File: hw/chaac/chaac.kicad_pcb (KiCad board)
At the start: 4 copper layers, 53 parts, among them J1 Battery, J2 TC2030-CTX, J3 UART, J4 windrain, Q1 Q_PMOS_GSD, SW1 RST, SW2 RST, U1 TPS7A0530PDBVT, U2 NRF52811-QFAA, U3 BMP280, U4 SHT3x-DIS, U5 E22-X00M22S, Y2 32.768kHz

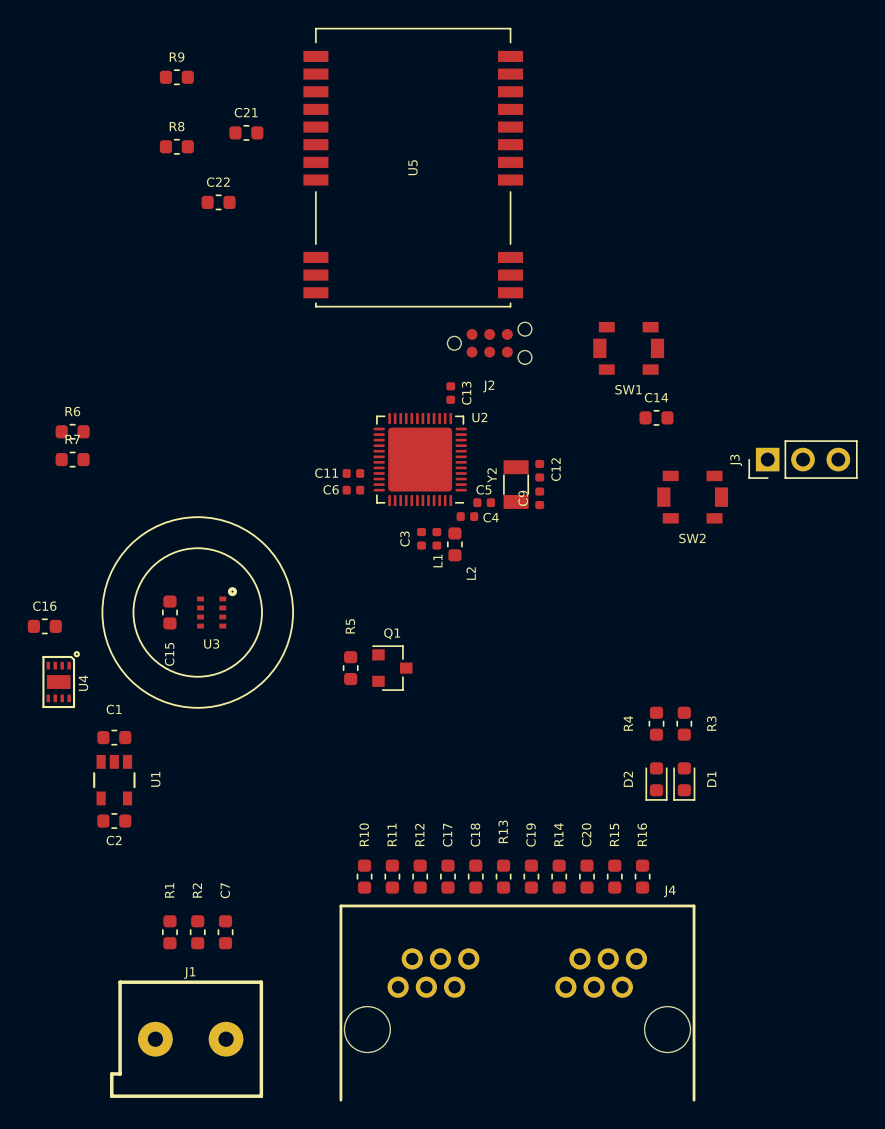
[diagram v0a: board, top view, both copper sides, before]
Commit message: Finished chaac v4.0!
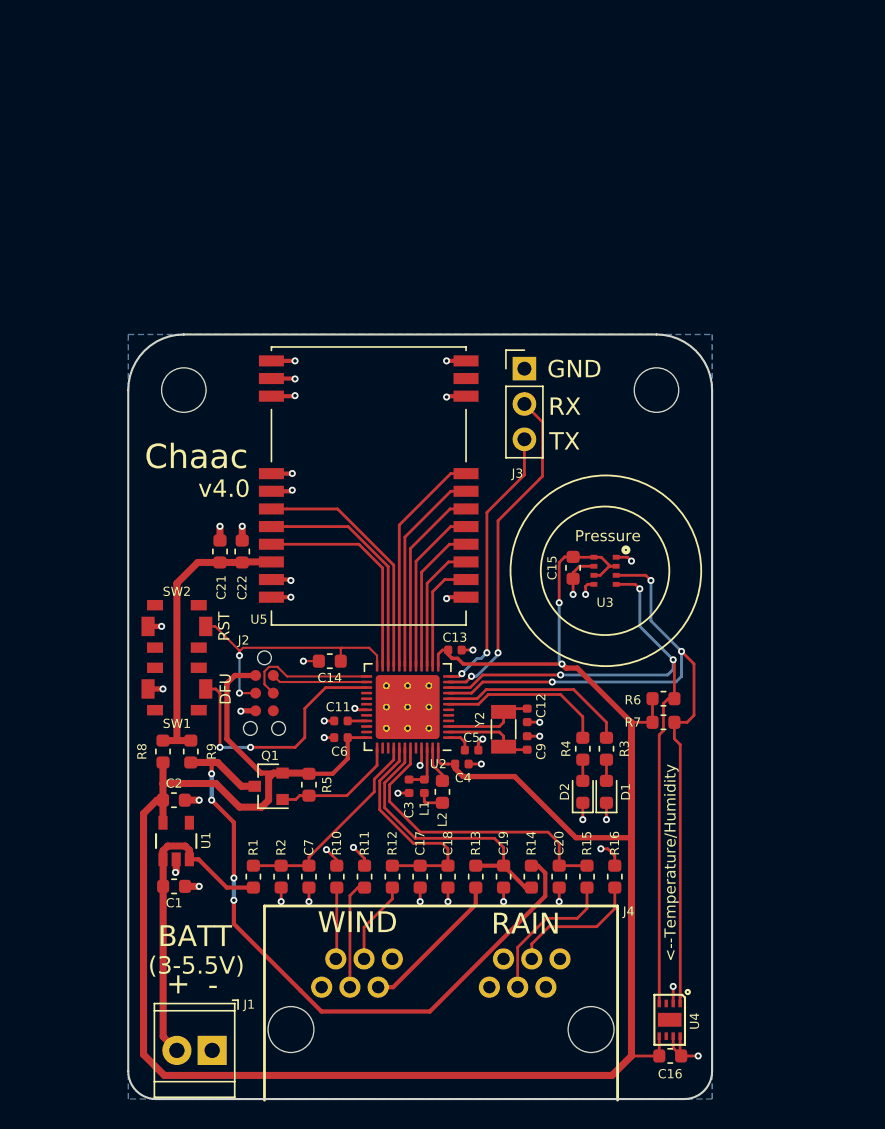
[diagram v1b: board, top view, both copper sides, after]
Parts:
- added REF**: OSHW-Logo_28.5x30mm_SilkScreen, Symbol:OSHW-Logo_28.5x30mm_SilkScreen, B.Cu at (124.4, 151.0)
- added REF**: MountingHole_3.2mm_M3, MountingHole:MountingHole_3.2mm_M3, F.Cu at (141.0, 133.0)
- added REF**: MountingHole_3.2mm_M3, MountingHole:MountingHole_3.2mm_M3, F.Cu at (107.0, 133.0)
- J1: footprint alvarop:‎282837-2‎ -> TerminalBlock_TE-Connectivity:TerminalBlock_TE_282834-2_1x02_P2.54mm_Horizontal
- U2: footprint alvarop:NRF52811-QFN48 -> alvarop:NRF52811-QFN48-VIAS
- moved C16 54.6 mm to (142.0, 180.9)
- moved U4 50.2 mm to (141.9, 178.3)
- moved R9 48.5 mm to (107.5, 159.0), turned to 270 degrees
- moved R6 46.6 mm to (141.5, 155.2), turned to 180 degrees
- moved R7 46.5 mm to (141.5, 156.9), turned to 180 degrees
- moved R8 43.5 mm to (105.5, 159.0), turned to 270 degrees
- moved SW1 40.7 mm to (106.5, 154.5)
- moved SW2 38.2 mm to (106.5, 150.0)
- moved C21 30.2 mm to (109.6, 144.6), turned to 90 degrees
- moved J2 29.9 mm to (112.8, 154.8), turned to 270 degrees
- moved C14 29.3 mm to (117.5, 152.5), turned to 180 degrees
- moved C15 29.2 mm to (135.0, 145.8)
- moved U3 28.5 mm to (137.3, 146.0)
- moved C22 25.2 mm to (111.2, 144.6), turned to 90 degrees
- moved J3 18.7 mm to (131.5, 131.5), turned to 0 degrees
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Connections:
- J1 pad 1: /VBATT -> GND
- J1 pad 2: GND -> /VBATT
- U2 pad 10: /UART_TX -> /SCL
- U2 pad 11: /LED1 -> /UART_RX
- U2 pad 12: /LED2 -> /UART_TX
- U2 pad 38: /RAIN -> Net-(U2-Pad38)
- U2 pad 39: /WSPEED -> Net-(U2-Pad39)
- U2 pad 40: /WDIR -> /BATT
- U2 pad 41: /BATT -> /WSPEED
- U2 pad 42: Net-(U2-Pad42) -> /WDIR
- U2 pad 43: Net-(U2-Pad43) -> /RAIN
- U2 pad 7: /SDA -> /LED2
- U2 pad 8: /SCL -> /LED1
- U2 pad 9: /UART_RX -> /SDA
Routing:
- net +3V3: track 0.00 -> 169.0 mm, vias 0 -> 2
- net GND: track 0.00 -> 58.2 mm, vias 0 -> 45
- net /SDA: track 0.00 -> 54.5 mm, vias 0 -> 3
- net /SCL: track 0.00 -> 50.6 mm, vias 0 -> 3
- net /SNS_3V3: track 0.00 -> 48.9 mm, vias 0 -> 4
- net /UART_RX: track 0.00 -> 24.3 mm, vias 0 -> 2
- net /VBATT: track 0.00 -> 23.0 mm
- net /RAIN: track 0.00 -> 21.5 mm
- net Net-(C21-Pad1): track 0.00 -> 20.7 mm
- net /WDIR: track 0.00 -> 20.6 mm
- net /UART_TX: track 0.00 -> 19.9 mm, vias 0 -> 2
- net /nRST: track 0.00 -> 19.4 mm, vias 0 -> 2
- net /BOOT: track 0.00 -> 18.6 mm, vias 0 -> 2
- net /E22_RXEN: track 0.00 -> 17.7 mm
- net /E22_TXEN: track 0.00 -> 16.7 mm
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- added copper zone on B.Cu, net GND
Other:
- board outline added: 42 x 55 mm
- copper layers 4 -> 2
- rule trace_min: 0.0889 -> 0.1524
- board text added: "(3-5.5V)"
- board text added: "+"
- board text added: "-"
- board text added: "<--Temperature/Humidity"
- board text added: "BATT"
- board text added: "Chaac"
- board text added: "DFU"
- board text added: "GND"
- board text added: "Pressure"
- board text added: "RAIN"
- board text added: "RST"
- board text added: "RX"
- board text added: "TX"
- board text added: "WIND"
- board text added: "by @alvaroprieto"
- board text added: "https://chaac.network"
- board text added: "https://github.com/alvarop/chaac/"
- board text added: "v4.0"
